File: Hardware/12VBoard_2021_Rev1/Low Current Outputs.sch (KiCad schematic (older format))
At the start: 39 parts, among them U2 INA198, U3 LM2576S-12/NOPB, U4 LM2576S-12/NOPB, U5 LM2576S-12/NOPB, U6 LM2576S-12/NOPB

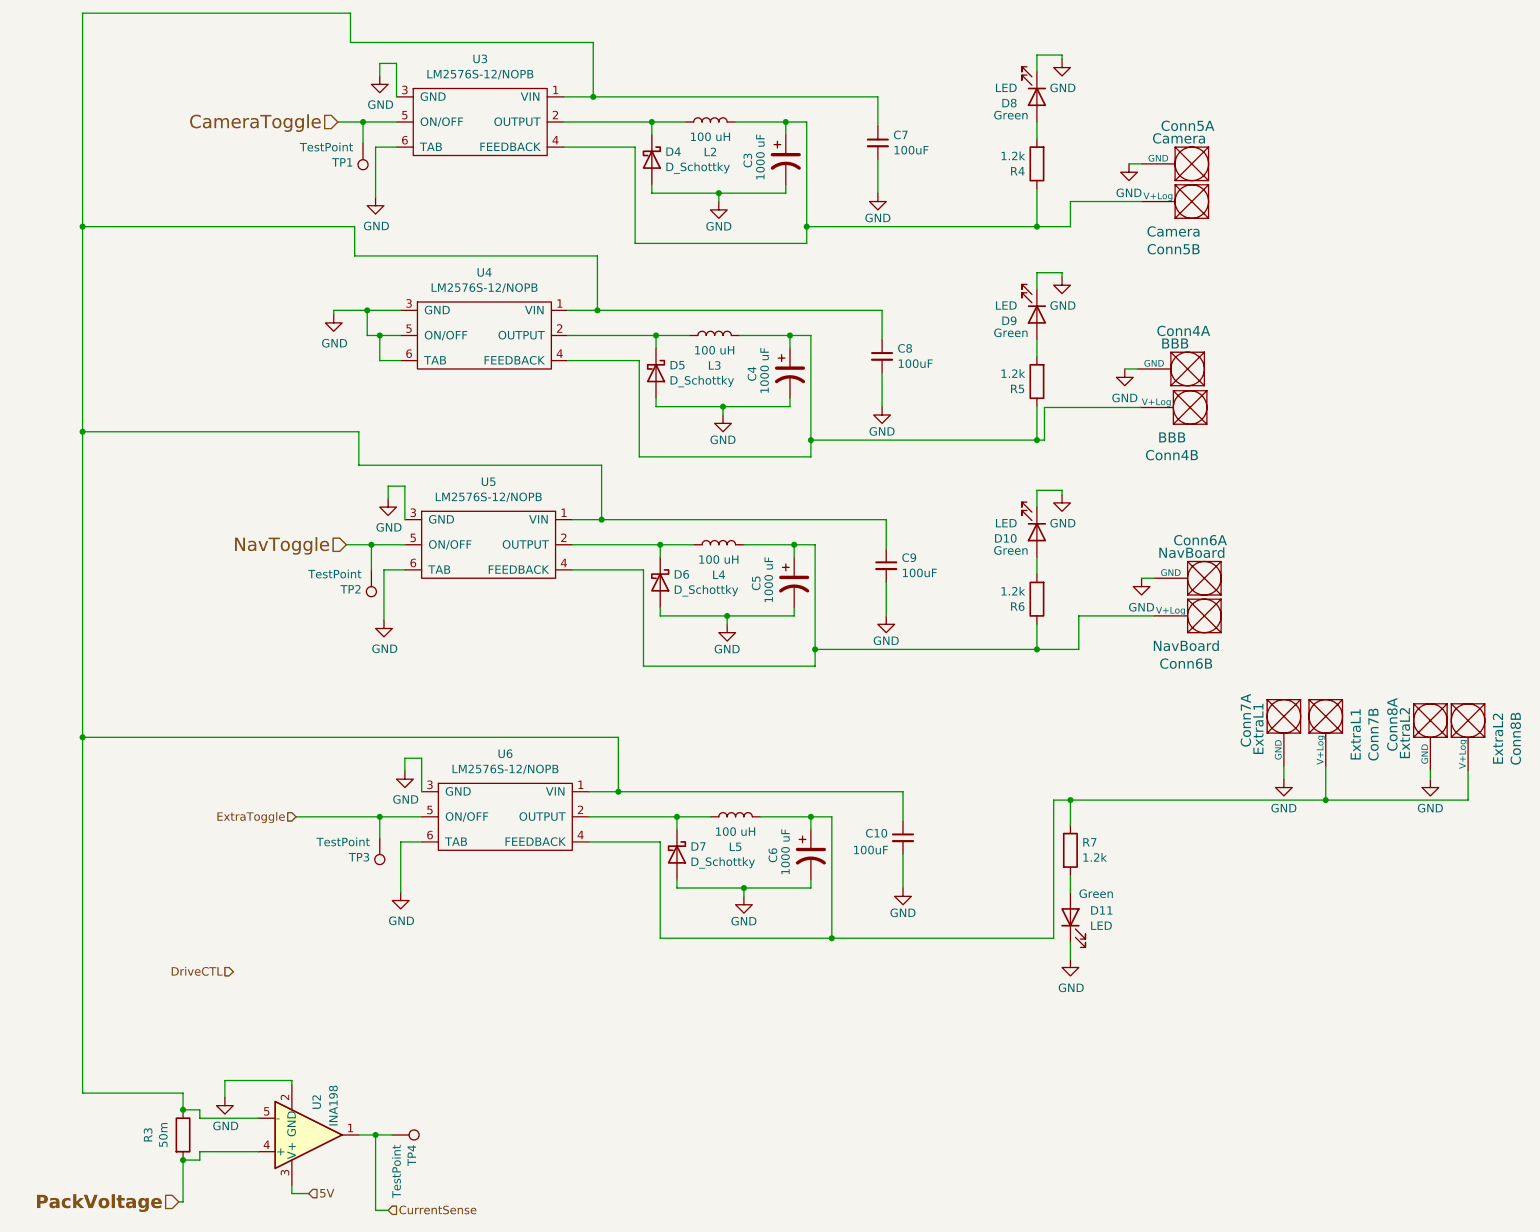
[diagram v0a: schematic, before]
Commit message: Layout Started
Board dimensions
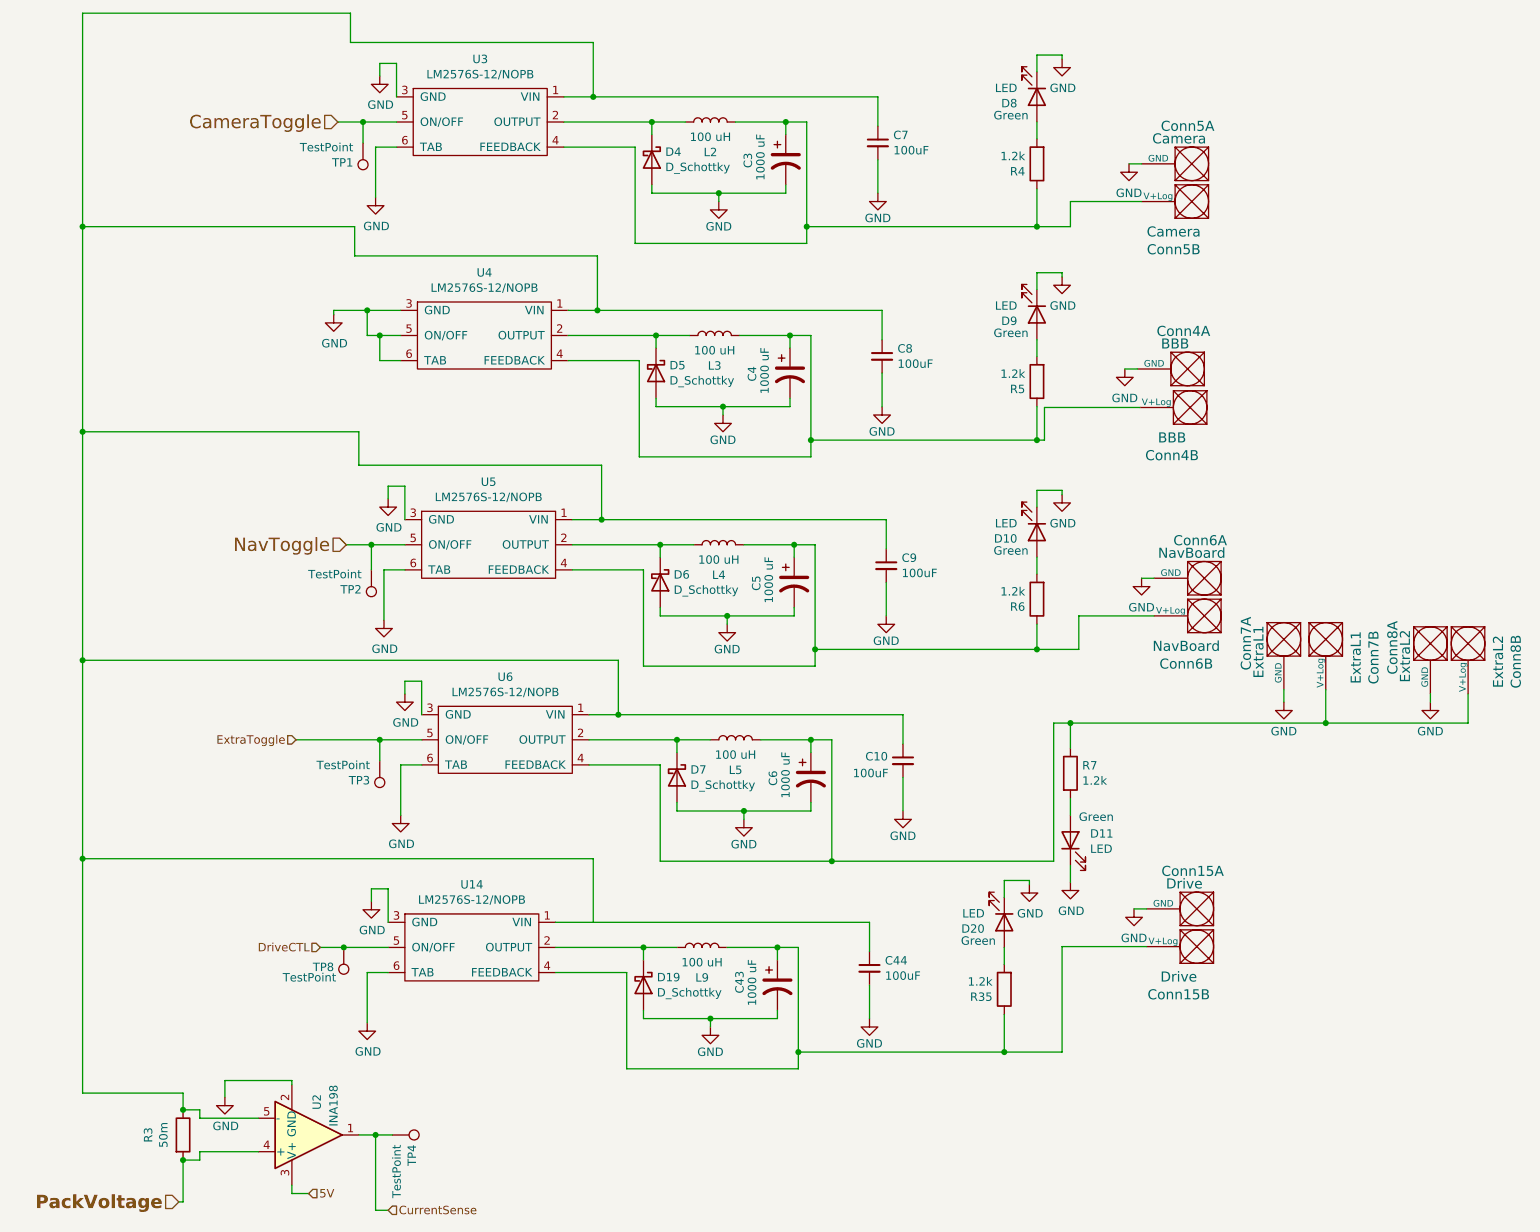
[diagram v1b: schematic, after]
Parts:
- added C43: 1000 uF, Capacitor_THT:CP_Axial_L20.0mm_D10.0mm_P26.00mm_Horizontal, symbol Device:CP1
- added C44: 100uF, Capacitor_SMD:C_0603_1608Metric_Pad1.05x0.95mm_HandSolder, symbol Device:C_Small
- added Conn15: Drive, MRDT_Connectors:Anderson_2_Horizontal_Stacked, symbol MRDT_Connectors:AndersonPP
- added D19: D_Schottky, Diode_SMD:D_0603_1608Metric_Pad1.05x0.95mm_HandSolder, symbol Device:D_Schottky
- added D20: LED, Diode_SMD:D_0603_1608Metric_Pad1.05x0.95mm_HandSolder, symbol Device:LED
- added L9: 100 uH, Inductor_SMD:L_0603_1608Metric_Pad1.05x0.95mm_HandSolder, symbol Device:L
- added R35: 1.2k, Resistor_SMD:R_0603_1608Metric_Pad1.05x0.95mm_HandSolder, symbol Device:R
- added TP8: TestPoint, TestPoint:TestPoint_Pad_2.5x2.5mm, symbol Connector:TestPoint
- added U14: LM2576S-12/NOPB, MRDT_Devices:LM2576, symbol 12VBoard_2021_Rev1-rescue:LM2576D2TR4-MRDT_Devices
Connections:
- net DriveCTL: now also TP8.1, U14.5 (ON/OFF)
- net GND: now also C43.2, C44.2, Conn15.1 (GND), D19.2 (A), D20.1 (K), U14.3 (GND), U14.6 (TAB)
- new net: D19.1 (K), L9.1, U14.2 (OUTPUT)
- new net: C43.1, Conn15.2 (V+Log), L9.2, R35.1, U14.4 (FEEDBACK)
- new net: C44.1, U14.1 (VIN)
- new net: D20.2 (A), R35.2
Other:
- moved on the sheet: C10, C6, Conn7A, Conn7B, Conn8A, Conn8B, D11, D7, L5, R7, TP3, U6
